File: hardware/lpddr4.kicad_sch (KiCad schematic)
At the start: 3 parts, among them IC11 K4F6E3S4HM-MGCJ, IC12 K4F6E3S4HM-MGCJ, U9 MPFS025T-FCVG484E

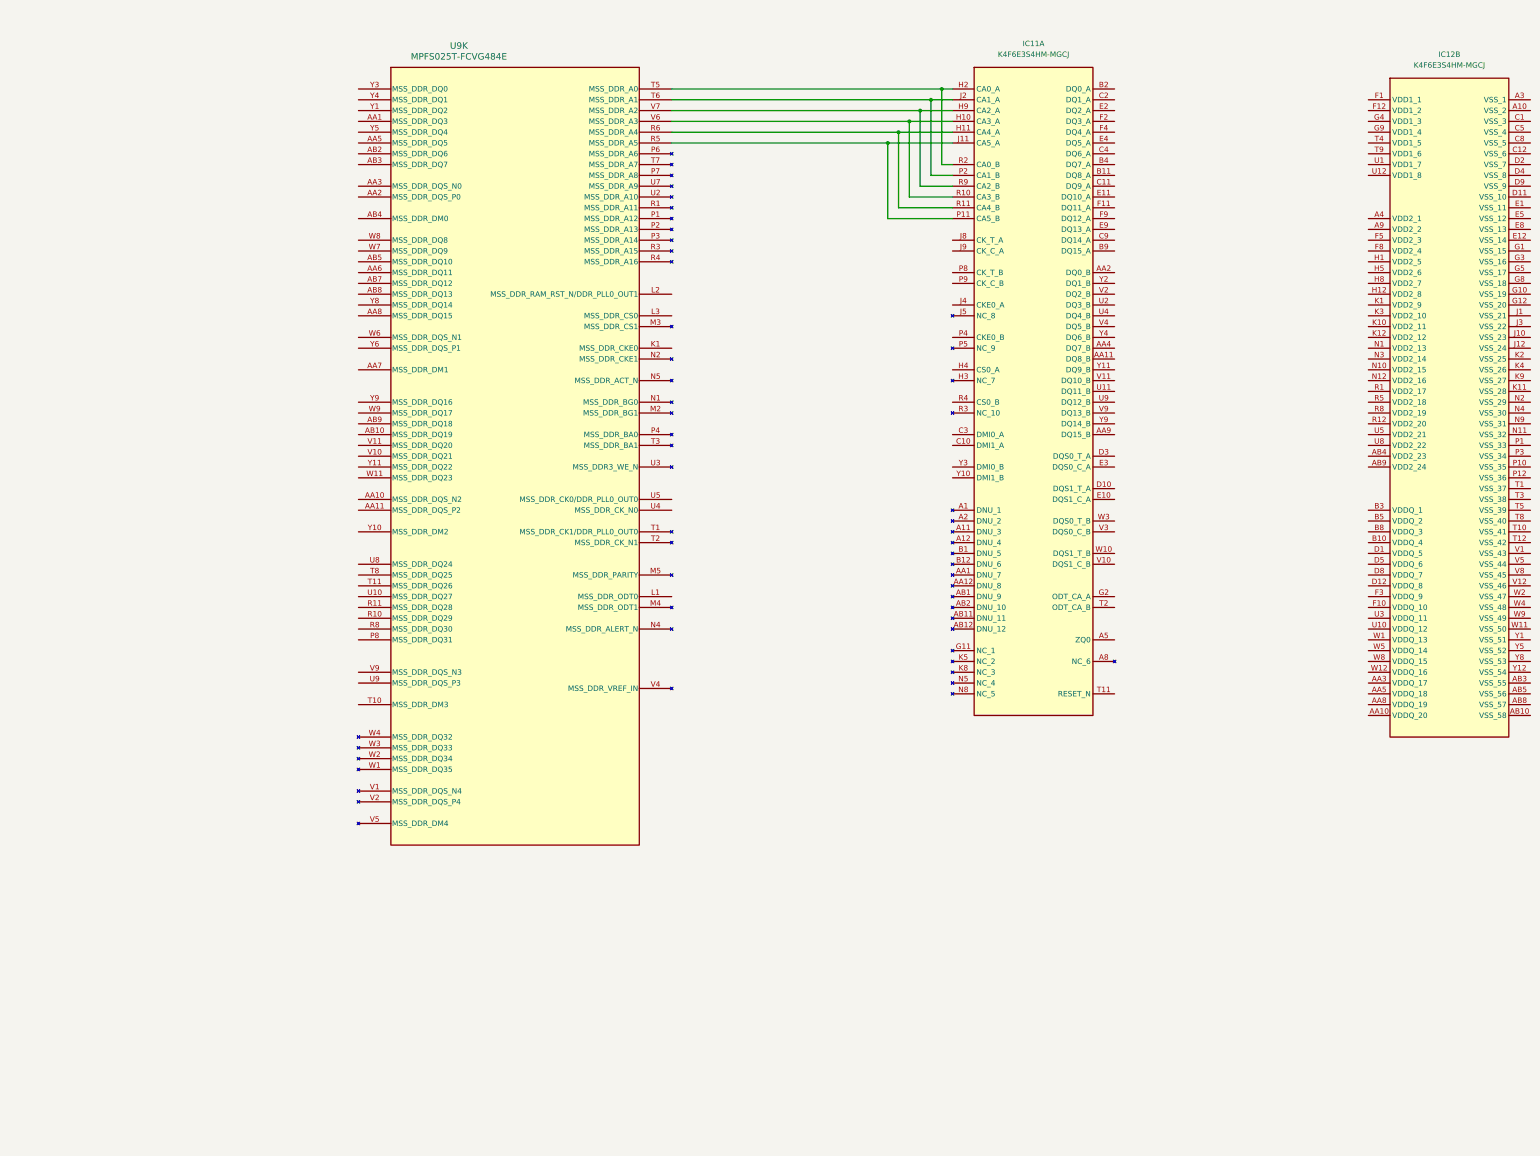
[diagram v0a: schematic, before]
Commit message: updated schematic
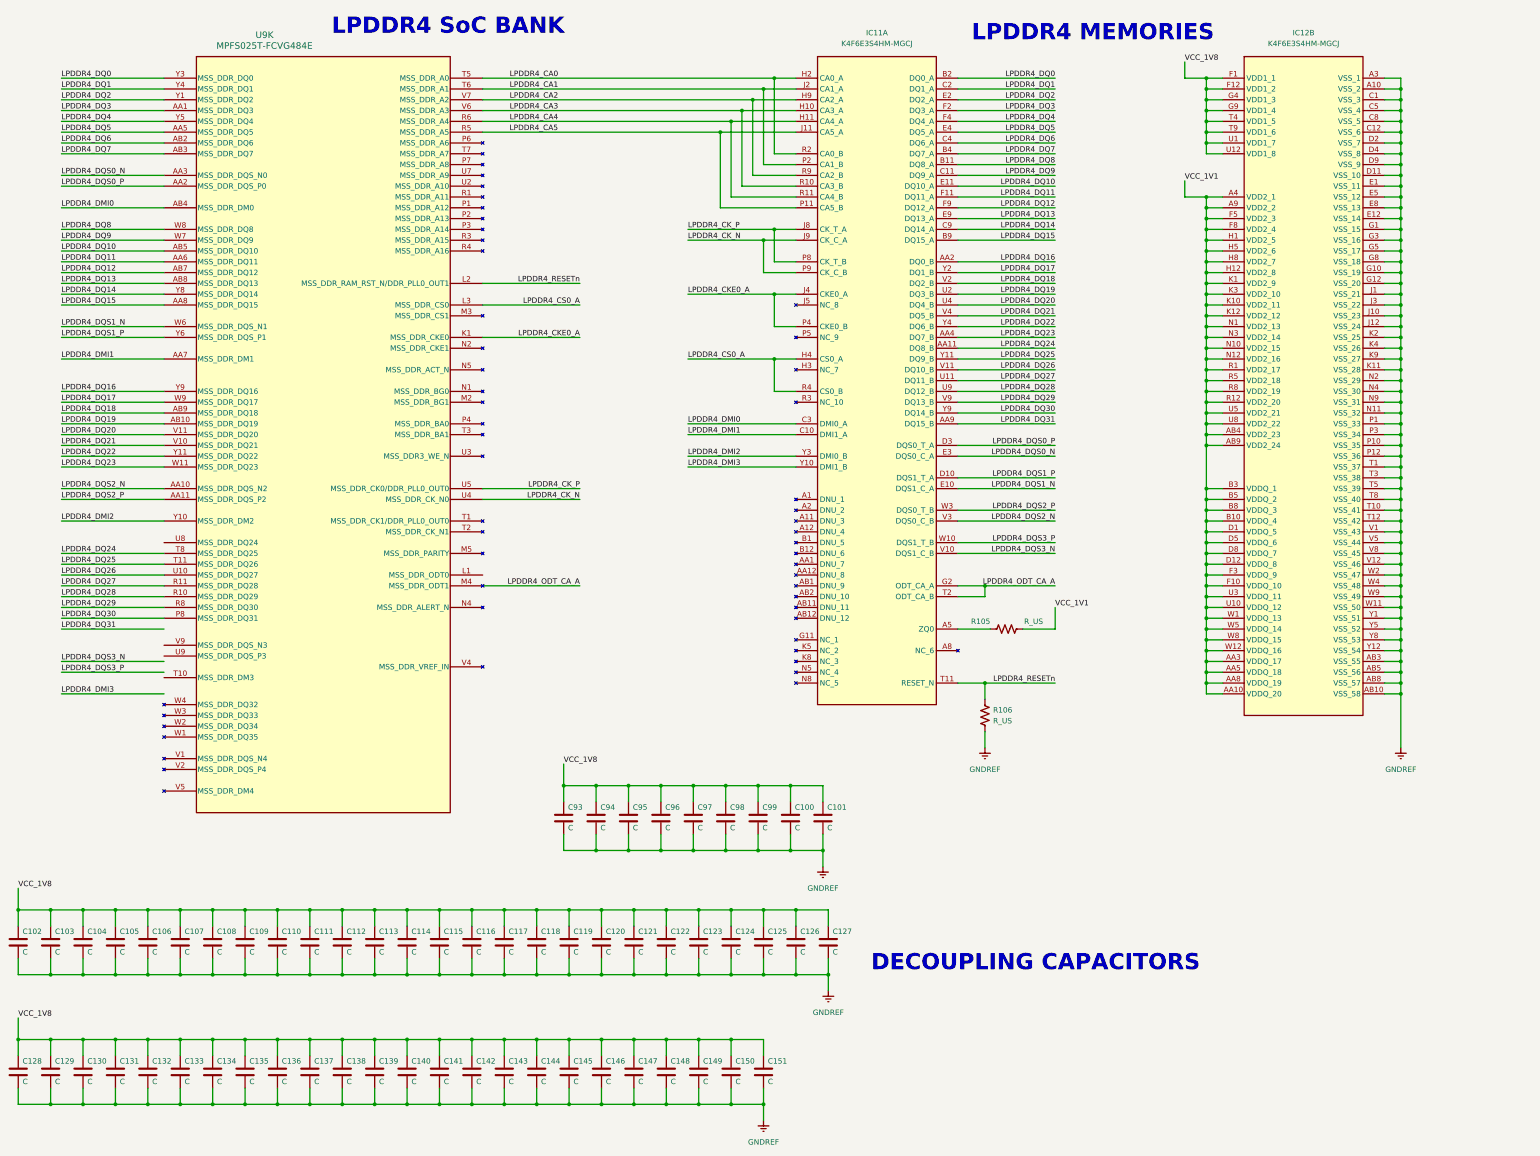
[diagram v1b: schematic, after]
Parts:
- added C100, C101, C102, C103, C104, C105, C106, C107, C108, C109, C110, C111, C112, C113, C114, C115, C116, C117, C118, C119, C120, C121, C122, C123, C124, C125, C126, C127, C128, C129, C130, C131, C132, C133, C134, C135, C136, C137, C138, C139, C140, C141, C142, C143, C144, C145, C146, C147, C148, C149, C150, C151, C93, C94, C95, C96, C97, C98, C99: C, symbol Device:C
- added R105, R106: R_US, symbol Device:R_US
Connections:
- net LPDDR4_DQ3: now reaches U9.AA1 (MSS_DDR_DQ3)
- net LPDDR4_DQ3: now also IC11.F2 (DQ3_A)
- net LPDDR4_DQS2_N: now reaches U9.AA10 (MSS_DDR_DQS_N2)
- net LPDDR4_DQS2_N: now also IC11.V3 (DQS0_C_B)
- net LPDDR4_DQS2_P: now reaches U9.AA11 (MSS_DDR_DQS_P2)
- net LPDDR4_DQS2_P: now also IC11.W3 (DQS0_T_B)
- net LPDDR4_DQS0_P: now reaches U9.AA2 (MSS_DDR_DQS_P0)
- net LPDDR4_DQS0_P: now also IC11.D3 (DQS0_T_A)
- net LPDDR4_DQS0_N: now reaches U9.AA3 (MSS_DDR_DQS_N0)
- net LPDDR4_DQS0_N: now also IC11.E3 (DQS0_C_A)
- net LPDDR4_DQ5: now reaches U9.AA5 (MSS_DDR_DQ5)
- net LPDDR4_DQ5: now also IC11.E4 (DQ5_A)
- net LPDDR4_DQ11: now reaches U9.AA6 (MSS_DDR_DQ11)
- net LPDDR4_DQ11: now also IC11.F11 (DQ11_A)
- net LPDDR4_DMI1: now reaches U9.AA7 (MSS_DDR_DM1)
- net LPDDR4_DMI1: now also IC11.C10 (DMI1_A)
- net LPDDR4_DQ15: now reaches U9.AA8 (MSS_DDR_DQ15)
- net LPDDR4_DQ15: now also IC11.B9 (DQ15_A)
- net LPDDR4_DQ19: now reaches U9.AB10 (MSS_DDR_DQ19)
- net LPDDR4_DQ19: now also IC11.U2 (DQ3_B)
- net LPDDR4_DQ6: now reaches U9.AB2 (MSS_DDR_DQ6)
- net LPDDR4_DQ6: now also IC11.C4 (DQ6_A)
- net LPDDR4_DQ7: now reaches U9.AB3 (MSS_DDR_DQ7)
- net LPDDR4_DQ7: now also IC11.B4 (DQ7_A)
- net LPDDR4_DMI0: now reaches U9.AB4 (MSS_DDR_DM0)
- net LPDDR4_DMI0: now also IC11.C3 (DMI0_A)
- net LPDDR4_DQ10: now reaches U9.AB5 (MSS_DDR_DQ10)
- net LPDDR4_DQ10: now also IC11.E11 (DQ10_A)
- net LPDDR4_DQ12: now reaches U9.AB7 (MSS_DDR_DQ12)
- net LPDDR4_DQ12: now also IC11.F9 (DQ12_A)
- net LPDDR4_DQ13: now reaches U9.AB8 (MSS_DDR_DQ13)
- net LPDDR4_DQ13: now also IC11.E9 (DQ13_A)
- net LPDDR4_DQ18: now reaches U9.AB9 (MSS_DDR_DQ18)
- net LPDDR4_DQ18: now also IC11.V2 (DQ2_B)
- net LPDDR4_CKE0_A: now reaches U9.K1 (MSS_DDR_CKE0)
- net LPDDR4_CKE0_A: now also IC11.J4 (CKE0_A), IC11.P4 (CKE0_B)
- net LPDDR4_RESETn: now reaches U9.L2 (MSS_DDR_RAM_RST_N/DDR_PLL0_OUT1)
- net LPDDR4_RESETn: now also IC11.T11 (RESET_N), R106.2
- net LPDDR4_CS0_A: now reaches U9.L3 (MSS_DDR_CS0)
- net LPDDR4_CS0_A: now also IC11.H4 (CS0_A), IC11.R4 (CS0_B)
- net LPDDR4_ODT_CA_A: now reaches U9.M4 (MSS_DDR_ODT1)
- net LPDDR4_ODT_CA_A: now also IC11.G2 (ODT_CA_A), IC11.T2 (ODT_CA_B)
- net LPDDR4_DQ30: now reaches U9.P8 (MSS_DDR_DQ31)
- net LPDDR4_DQ30: now also IC11.Y9 (DQ14_B)
- net LPDDR4_DQ28: now reaches U9.R10 (MSS_DDR_DQ29)
- net LPDDR4_DQ28: now also IC11.U9 (DQ12_B)
- net LPDDR4_DQ27: now reaches U9.R11 (MSS_DDR_DQ28)
- net LPDDR4_DQ27: now also IC11.U11 (DQ11_B)
- net LPDDR4_CA5: now reaches IC11.J11 (CA5_A), IC11.P11 (CA5_B), U9.R5 (MSS_DDR_A5)
- net LPDDR4_CA4: now reaches IC11.H11 (CA4_A), IC11.R11 (CA4_B), U9.R6 (MSS_DDR_A4)
- net LPDDR4_DQ29: now reaches U9.R8 (MSS_DDR_DQ30)
- net LPDDR4_DQ29: now also IC11.V9 (DQ13_B)
- net LPDDR4_DQ25: now reaches U9.T11 (MSS_DDR_DQ26)
- net LPDDR4_DQ25: now also IC11.Y11 (DQ9_B)
- net LPDDR4_CA0: now reaches IC11.H2 (CA0_A), IC11.R2 (CA0_B), U9.T5 (MSS_DDR_A0)
- net LPDDR4_CA1: now reaches IC11.J2 (CA1_A), IC11.P2 (CA1_B), U9.T6 (MSS_DDR_A1)
- net LPDDR4_DQ24: now reaches U9.T8 (MSS_DDR_DQ25)
- net LPDDR4_DQ24: now also IC11.AA11 (DQ8_B)
- net LPDDR4_DQ26: now reaches U9.U10 (MSS_DDR_DQ27)
- net LPDDR4_DQ26: now also IC11.V11 (DQ10_B)
- net LPDDR4_CK_N: now reaches U9.U4 (MSS_DDR_CK_N0)
- net LPDDR4_CK_N: now also IC11.J9 (CK_C_A), IC11.P9 (CK_C_B)
- net LPDDR4_CK_P: now reaches U9.U5 (MSS_DDR_CK0/DDR_PLL0_OUT0)
- net LPDDR4_CK_P: now also IC11.J8 (CK_T_A), IC11.P8 (CK_T_B)
- net LPDDR4_DQ21: now reaches U9.V10 (MSS_DDR_DQ21)
- net LPDDR4_DQ21: now also IC11.V4 (DQ5_B)
- net LPDDR4_DQ20: now reaches U9.V11 (MSS_DDR_DQ20)
- net LPDDR4_DQ20: now also IC11.U4 (DQ4_B)
- net LPDDR4_CA3: now reaches IC11.H10 (CA3_A), IC11.R10 (CA3_B), U9.V6 (MSS_DDR_A3)
- net LPDDR4_CA2: now reaches IC11.H9 (CA2_A), IC11.R9 (CA2_B), U9.V7 (MSS_DDR_A2)
- net LPDDR4_DQ23: now reaches U9.W11 (MSS_DDR_DQ23)
- net LPDDR4_DQ23: now also IC11.AA4 (DQ7_B)
- net LPDDR4_DQS1_N: now reaches U9.W6 (MSS_DDR_DQS_N1)
- net LPDDR4_DQS1_N: now also IC11.E10 (DQS1_C_A)
- net LPDDR4_DQ9: now reaches U9.W7 (MSS_DDR_DQ9)
- net LPDDR4_DQ9: now also IC11.C11 (DQ9_A)
- net LPDDR4_DQ8: now reaches U9.W8 (MSS_DDR_DQ8)
- net LPDDR4_DQ8: now also IC11.B11 (DQ8_A)
- net LPDDR4_DQ17: now reaches U9.W9 (MSS_DDR_DQ17)
- net LPDDR4_DQ17: now also IC11.Y2 (DQ1_B)
- net LPDDR4_DQ2: now reaches U9.Y1 (MSS_DDR_DQ2)
- net LPDDR4_DQ2: now also IC11.E2 (DQ2_A)
- net LPDDR4_DMI2: now reaches U9.Y10 (MSS_DDR_DM2)
- net LPDDR4_DMI2: now also IC11.Y3 (DMI0_B)
- net LPDDR4_DQ22: now reaches U9.Y11 (MSS_DDR_DQ22)
- net LPDDR4_DQ22: now also IC11.Y4 (DQ6_B)
- net LPDDR4_DQ0: now reaches U9.Y3 (MSS_DDR_DQ0)
- net LPDDR4_DQ0: now also IC11.B2 (DQ0_A)
- net LPDDR4_DQ1: now reaches U9.Y4 (MSS_DDR_DQ1)
- net LPDDR4_DQ1: now also IC11.C2 (DQ1_A)
- net LPDDR4_DQ4: now reaches U9.Y5 (MSS_DDR_DQ4)
- net LPDDR4_DQ4: now also IC11.F4 (DQ4_A)
- net LPDDR4_DQS1_P: now reaches U9.Y6 (MSS_DDR_DQS_P1)
- net LPDDR4_DQS1_P: now also IC11.D10 (DQS1_T_A)
- net LPDDR4_DQ14: now reaches U9.Y8 (MSS_DDR_DQ14)
- net LPDDR4_DQ14: now also IC11.C9 (DQ14_A)
- net LPDDR4_DQ16: now reaches U9.Y9 (MSS_DDR_DQ16)
- net LPDDR4_DQ16: now also IC11.AA2 (DQ0_B)
- net GNDREF: now reaches IC12.A10 (VSS_2)
- net GNDREF: now also IC12.A3 (VSS_1), IC12.AB10 (VSS_58), IC12.AB3 (VSS_55), IC12.AB5 (VSS_56), IC12.AB8 (VSS_57), IC12.C1 (VSS_3), IC12.C12 (VSS_6), IC12.C5 (VSS_4), IC12.C8 (VSS_5), IC12.D11 (VSS_10), IC12.D2 (VSS_7), IC12.D4 (VSS_8), IC12.D9 (VSS_9), IC12.E1 (VSS_11), IC12.E12 (VSS_14), IC12.E5 (VSS_12), IC12.E8 (VSS_13), IC12.G1 (VSS_15), IC12.G10 (VSS_19), IC12.G12 (VSS_20), IC12.G3 (VSS_16), IC12.G5 (VSS_17), IC12.G8 (VSS_18), IC12.J1 (VSS_21), IC12.J10 (VSS_23), IC12.J12 (VSS_24), IC12.J3 (VSS_22), IC12.K11 (VSS_28), IC12.K2 (VSS_25), IC12.K4 (VSS_26), IC12.K9 (VSS_27), IC12.N11 (VSS_32), IC12.N2 (VSS_29), IC12.N4 (VSS_30), IC12.N9 (VSS_31), IC12.P1 (VSS_33), IC12.P10 (VSS_35), IC12.P12 (VSS_36), IC12.P3 (VSS_34), IC12.T1 (VSS_37), IC12.T10 (VSS_41), IC12.T12 (VSS_42), IC12.T3 (VSS_38), IC12.T5 (VSS_39), IC12.T8 (VSS_40), IC12.V1 (VSS_43), IC12.V12 (VSS_46), IC12.V5 (VSS_44), IC12.V8 (VSS_45), IC12.W11 (VSS_50), IC12.W2 (VSS_47), IC12.W4 (VSS_48), IC12.W9 (VSS_49), IC12.Y1 (VSS_51), IC12.Y12 (VSS_54), IC12.Y5 (VSS_52), IC12.Y8 (VSS_53), C100.1, C101.1, C102.1, C103.1, C104.1, C105.1, C106.1, C107.1, C108.1, C109.1, C110.1, C111.1, C112.1, C113.1, C114.1, C115.1, C116.1, C117.1, C118.1, C119.1, C120.1, C121.1, C122.1, C123.1, C124.1, C125.1, C126.1, C127.1, C128.1, C129.1, C130.1, C131.1, C132.1, C133.1, C134.1, C135.1, C136.1, C137.1, C138.1, C139.1, C140.1, C141.1, C142.1, C143.1, C144.1, C145.1, C146.1, C147.1, C148.1, C149.1, C150.1, C151.1, C93.1, C94.1, C95.1, C96.1, C97.1, C98.1, C99.1, R106.1
- net VCC_1V1: now reaches IC12.A4 (VDD2_1)
- net VCC_1V1: now also IC12.A9 (VDD2_2), IC12.AA10 (VDDQ_20), IC12.AA3 (VDDQ_17), IC12.AA5 (VDDQ_18), IC12.AA8 (VDDQ_19), IC12.AB4 (VDD2_23), IC12.AB9 (VDD2_24), IC12.B10 (VDDQ_4), IC12.B3 (VDDQ_1), IC12.B5 (VDDQ_2), IC12.B8 (VDDQ_3), IC12.D1 (VDDQ_5), IC12.D12 (VDDQ_8), IC12.D5 (VDDQ_6), IC12.D8 (VDDQ_7), IC12.F10 (VDDQ_10), IC12.F3 (VDDQ_9), IC12.F5 (VDD2_3), IC12.F8 (VDD2_4), IC12.H1 (VDD2_5), IC12.H12 (VDD2_8), IC12.H5 (VDD2_6), IC12.H8 (VDD2_7), IC12.K1 (VDD2_9), IC12.K10 (VDD2_11), IC12.K12 (VDD2_12), IC12.K3 (VDD2_10), IC12.N1 (VDD2_13), IC12.N10 (VDD2_15), IC12.N12 (VDD2_16), IC12.N3 (VDD2_14), IC12.R1 (VDD2_17), IC12.R12 (VDD2_20), IC12.R5 (VDD2_18), IC12.R8 (VDD2_19), IC12.U10 (VDDQ_12), IC12.U3 (VDDQ_11), IC12.U5 (VDD2_21), IC12.U8 (VDD2_22), IC12.W1 (VDDQ_13), IC12.W12 (VDDQ_16), IC12.W5 (VDDQ_14), IC12.W8 (VDDQ_15), R105.2
- net VCC_1V8: now reaches IC12.F1 (VDD1_1)
- net VCC_1V8: now also IC12.F12 (VDD1_2), IC12.G4 (VDD1_3), IC12.G9 (VDD1_4), IC12.T4 (VDD1_5), IC12.T9 (VDD1_6), IC12.U1 (VDD1_7), IC12.U12 (VDD1_8), C100.2, C101.2, C102.2, C103.2, C104.2, C105.2, C106.2, C107.2, C108.2, C109.2, C110.2, C111.2, C112.2, C113.2, C114.2, C115.2, C116.2, C117.2, C118.2, C119.2, C120.2, C121.2, C122.2, C123.2, C124.2, C125.2, C126.2, C127.2, C128.2, C129.2, C130.2, C131.2, C132.2, C133.2, C134.2, C135.2, C136.2, C137.2, C138.2, C139.2, C140.2, C141.2, C142.2, C143.2, C144.2, C145.2, C146.2, C147.2, C148.2, C149.2, C150.2, C151.2, C93.2, C94.2, C95.2, C96.2, C97.2, C98.2, C99.2
- net at IC11.A5 (ZQ0): now also R105.1
- net LPDDR4_DQ31: now reaches IC11.AA9 (DQ15_B)
- net LPDDR4_DQS3_N: now reaches IC11.V10 (DQS1_C_B)
- net LPDDR4_DQS3_P: now reaches IC11.W10 (DQS1_T_B)
- net LPDDR4_DMI3: now reaches IC11.Y10 (DMI1_B)
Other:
- note added: "DECOUPLING CAPACITORS"
- note added: "LPDDR4 MEMORIES"
- note added: "LPDDR4 SoC BANK"
- moved on the sheet: IC11A, IC12B, U9K
